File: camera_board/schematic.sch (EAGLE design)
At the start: 6 parts

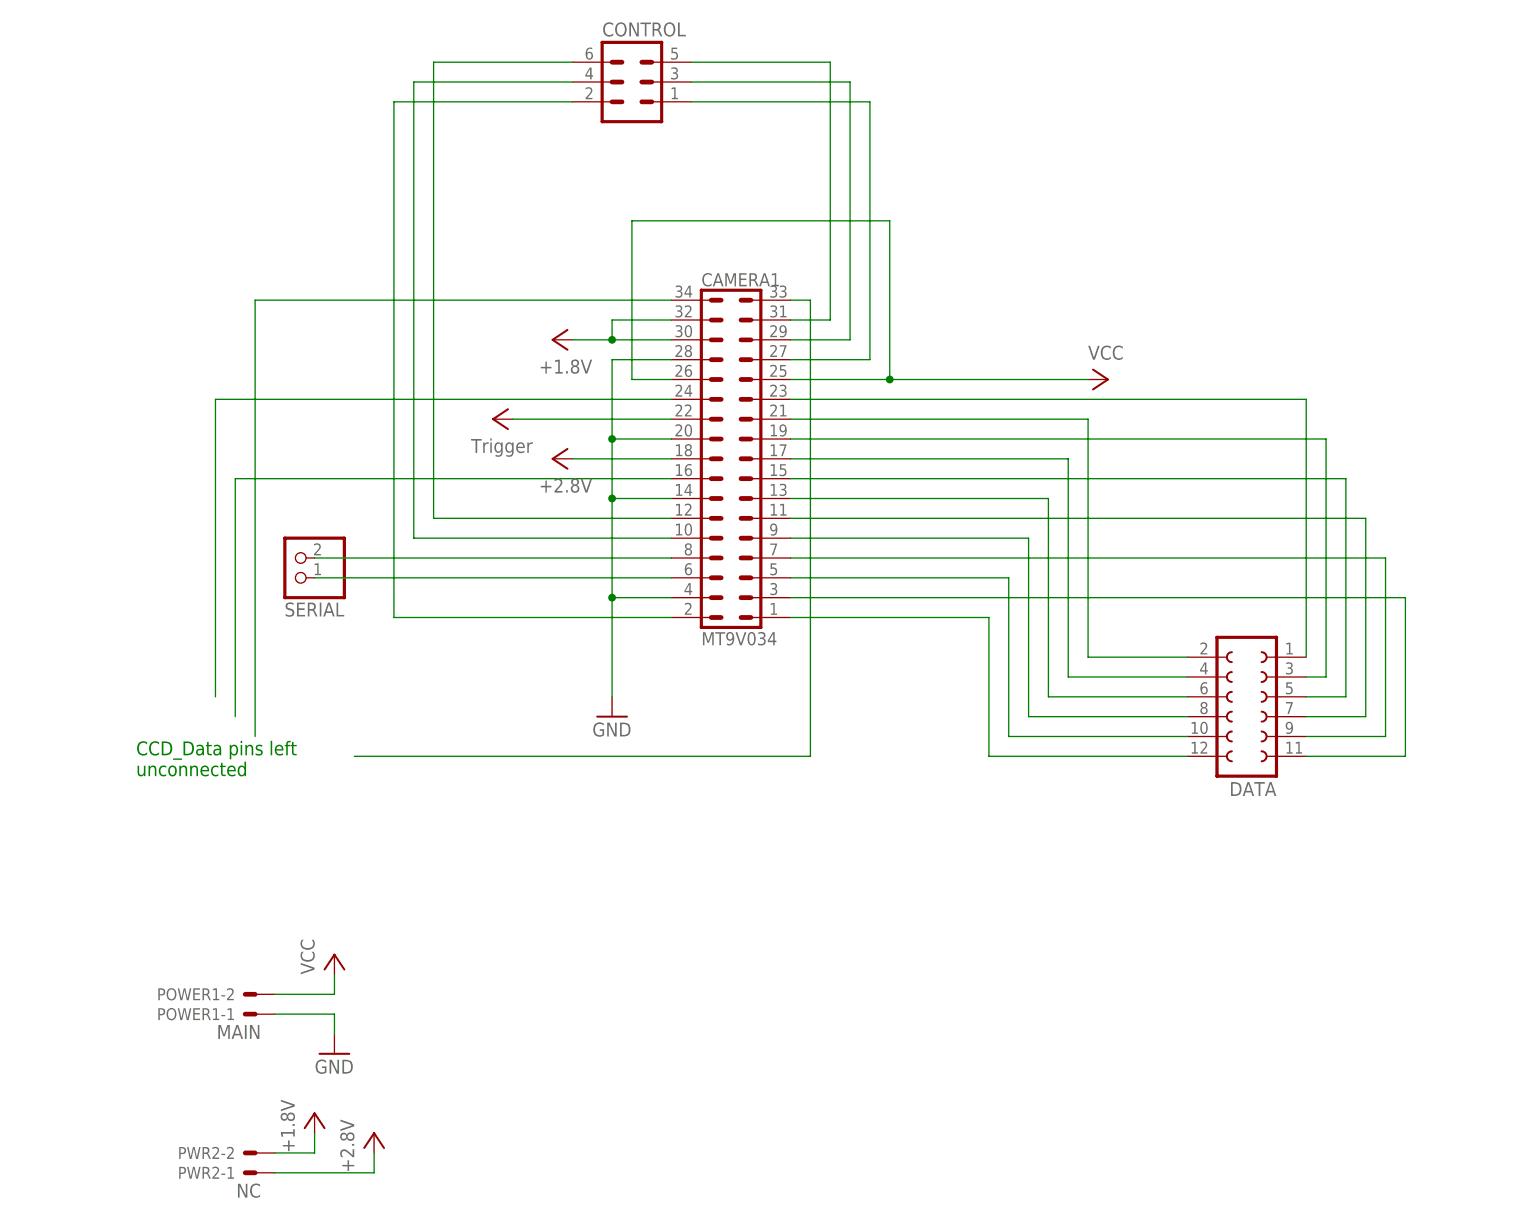
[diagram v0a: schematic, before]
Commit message: Final Schematic Part II
Need to double check and then I'll order boards
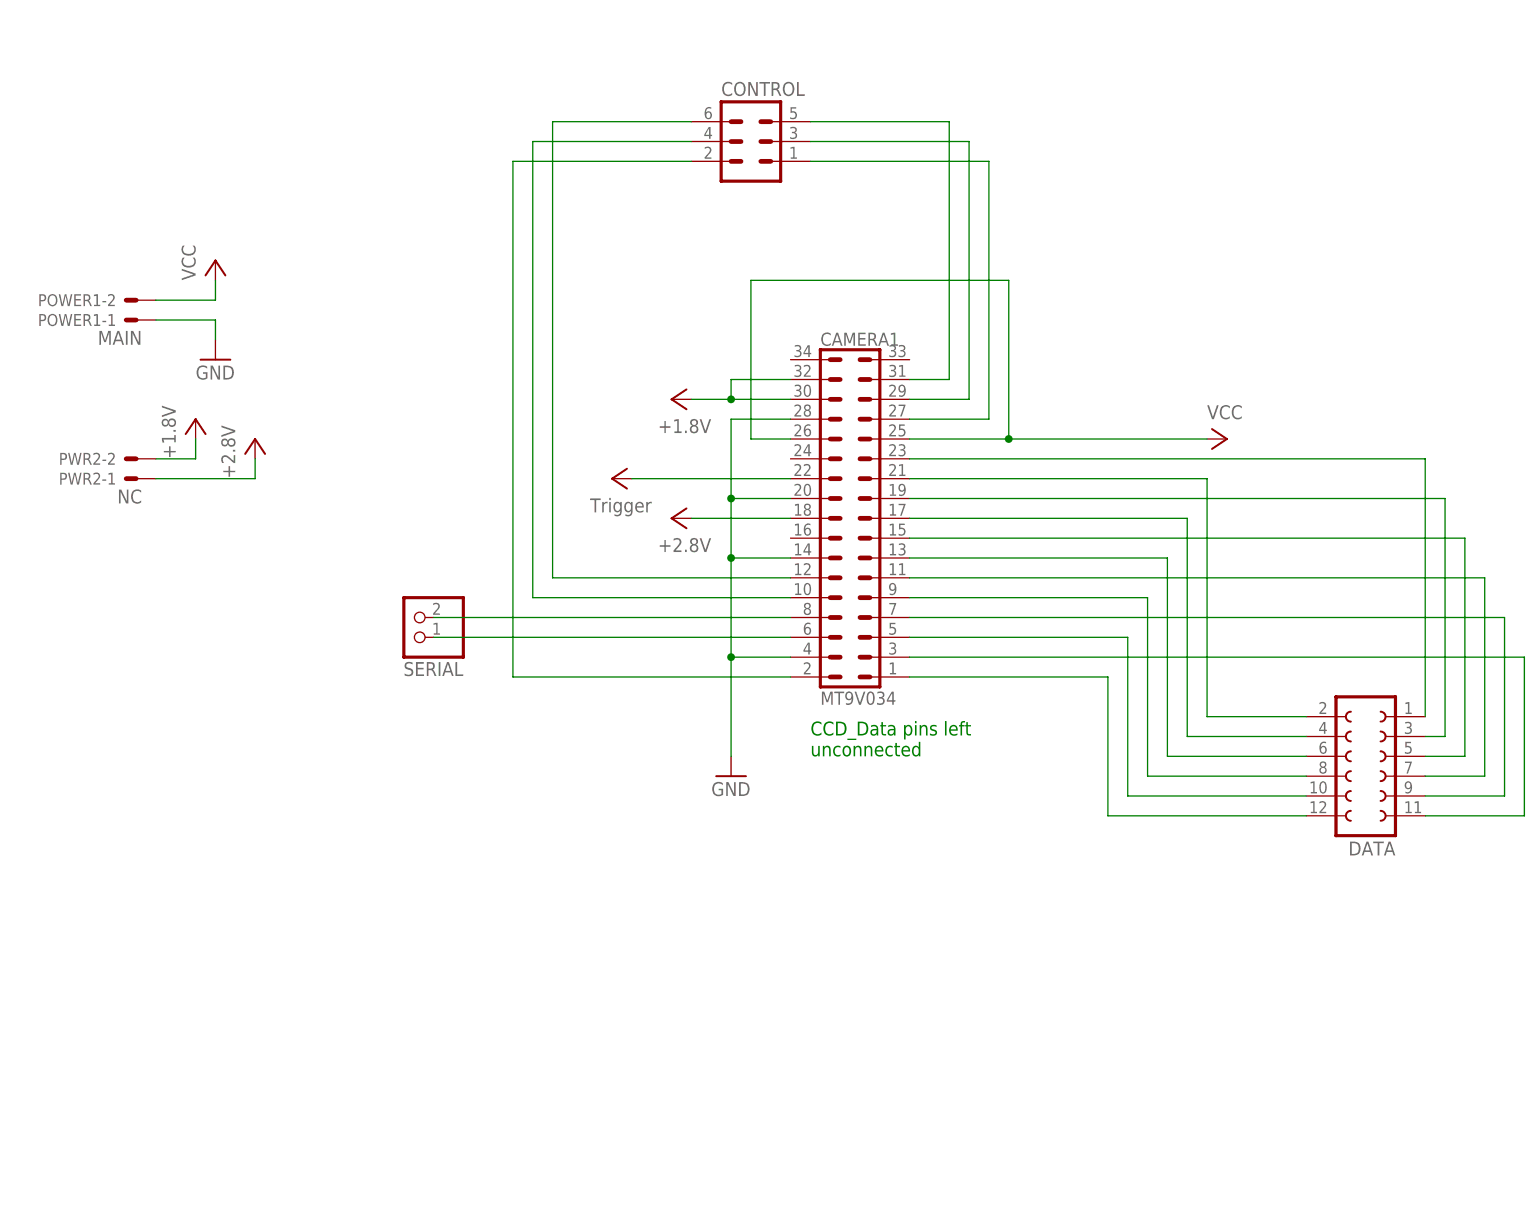
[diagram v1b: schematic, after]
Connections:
- removed net N$19: CAMERA1.33
- removed net N$20: CAMERA1.34
- removed net N$21: CAMERA1.16
- removed net N$22: CAMERA1.24
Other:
- moved on the sheet: CAMERA1, CONTROL, DATA, POWER1-1, POWER1-2, PWR2-1, PWR2-2, SERIAL
